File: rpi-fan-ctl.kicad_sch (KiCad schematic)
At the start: 21 parts, among them J2 Conn_01x05, Q4 NPN, U1 74LVC2G17, U2 74LVC2G17, U3 74LVC2G17

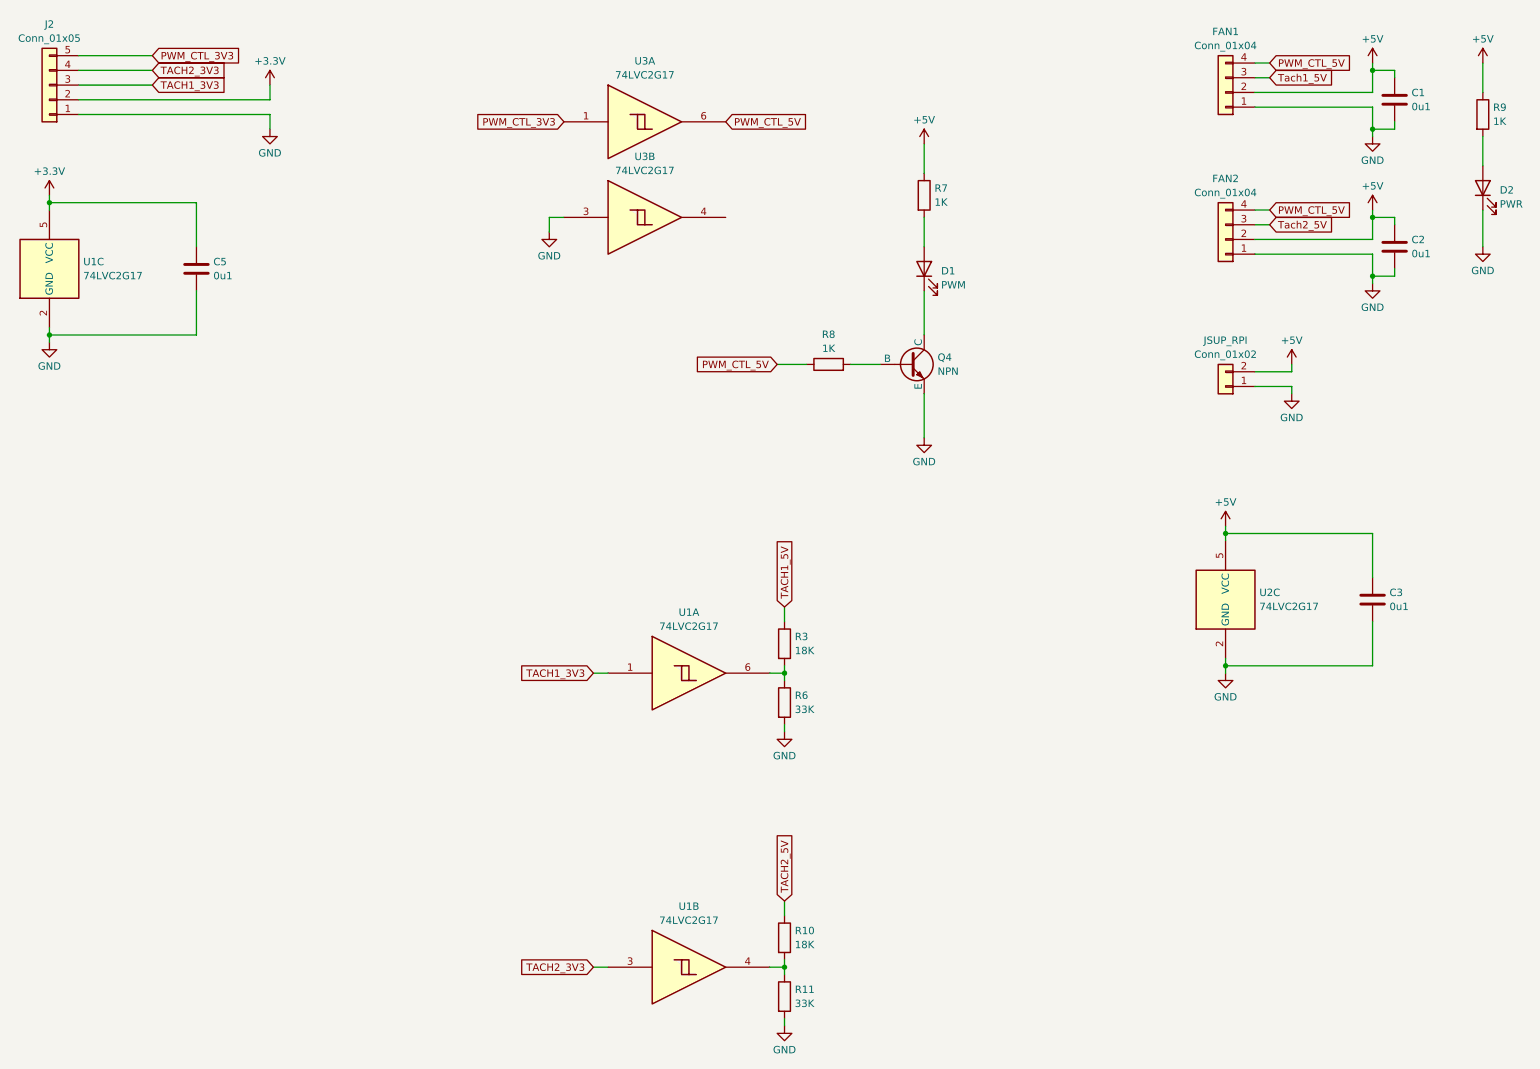
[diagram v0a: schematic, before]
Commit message: some routing progress
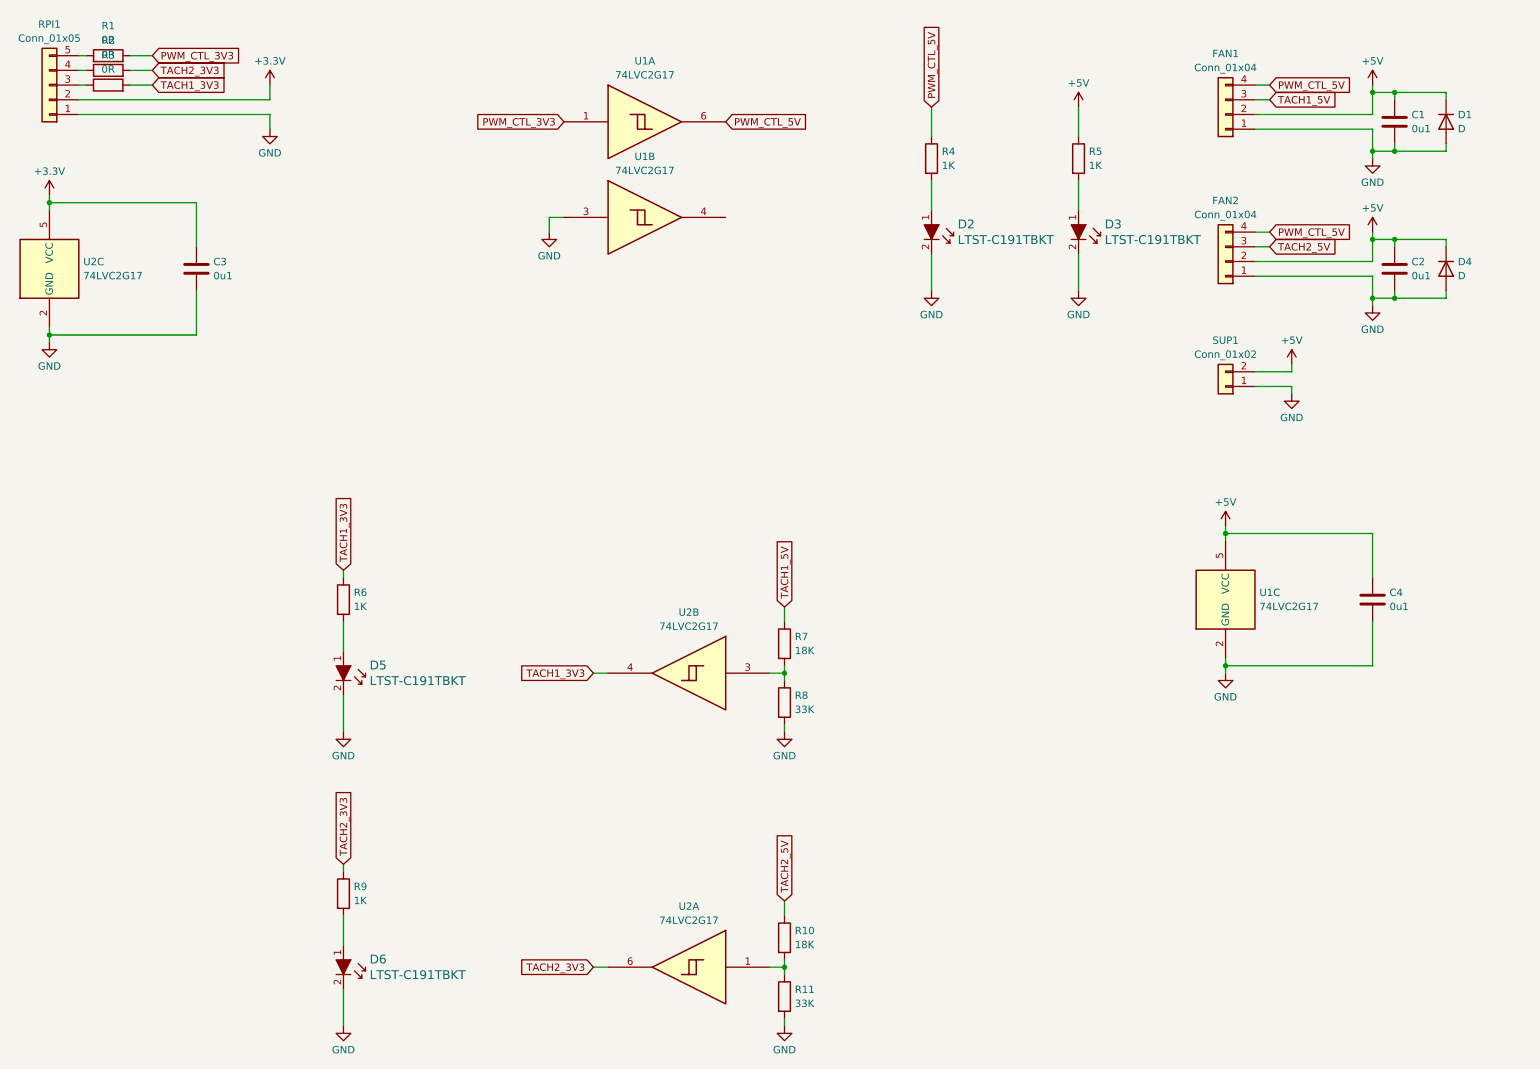
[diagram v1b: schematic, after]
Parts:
- removed D1: PWM, symbol Device:LED
- removed D2: PWR, symbol Device:LED
- removed Q4: NPN, symbol Simulation_SPICE:NPN
- removed R8: 1K, Resistor_SMD:R_0603_1608Metric_Pad0.98x0.95mm_HandSolder, symbol Device:R
- added D1: D, Diode_SMD:D_SOD-123F, symbol Device:D
- added D2, D3, D5, D6: LTST-C191TBKT, Diode_SMD:D_0402_1005Metric_Pad0.77x0.64mm_HandSolder, symbol J-Link-SWD-rescue:LTST-C191TBKT-dk_LED-Indication-Discrete
- added D4: D, Diode_SMD:D_SOD-123, symbol Device:D
- added R1, R2, R3: 0R, Resistor_SMD:R_0603_1608Metric_Pad0.98x0.95mm_HandSolder, symbol Device:R
- added R6, R9: 1K, Resistor_SMD:R_0603_1608Metric_Pad0.98x0.95mm_HandSolder, symbol Device:R
- FAN1, FAN2: footprint (none) -> Connector_PinHeader_2.54mm:PinHeader_1x04_P2.54mm_Horizontal
- RPI1: renamed from J2; footprint (none) -> Connector_PinHeader_2.54mm:PinHeader_1x05_P2.54mm_Vertical
- SUP1: renamed from JSUP_RPI; footprint (none) -> Connector_PinHeader_2.54mm:PinHeader_1x02_P2.54mm_Horizontal
- U1: renamed from U3; footprint Package_TO_SOT_SMD:SOT-363_SC-70-6_Handsoldering -> Package_TO_SOT_SMD:SOT-23-6_Handsoldering; DigiKey https://www.digikey.de/en/products/detail/texas-instruments/SN74LVC2G17DCKR/479737 -> https://www.digikey.de/en/products/detail/texas-instruments/SN74LVC2G17DBVR/479735
- U1: renamed from U2; footprint (none) -> Package_TO_SOT_SMD:SOT-23-6_Handsoldering; DigiKey (none) -> https://www.digikey.de/en/products/detail/texas-instruments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
- U2: renamed from U1; footprint Package_TO_SOT_SMD:SOT-363_SC-70-6_Handsoldering -> Package_TO_SOT_SMD:SOT-23-6_Handsoldering; DigiKey https://www.digikey.de/en/products/detail/texas-instruments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 -> (none)
- U2: renamed from U1; footprint (none) -> Package_TO_SOT_SMD:SOT-23-6_Handsoldering
- renumbered C5 to C3, C3 to C4, R7 to R4, R9 to R5, R3 to R7, R6 to R8
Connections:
- net Tach1_5V is gone; now on net TACH1_5V: FAN1.3 (Pin_3)
- net Tach2_5V is gone; now on net TACH2_5V: FAN2.3 (Pin_3)
- net +5V: now also D1.1 (K), D4.1 (K); no longer R4.1
- net GND: now also D1.2 (A), D2.2, D3.2, D4.2 (A), D5.2, D6.2
- net PWM_CTL_3V3: now also R1.2; no longer RPI1.5 (Pin_5)
- net PWM_CTL_5V: now also R4.1
- net TACH1_3V3: now also U2.4, R3.2, R6.1; no longer RPI1.3 (Pin_3), U2.1
- net TACH2_3V3: now also U2.6, R2.2, R9.1; no longer RPI1.4 (Pin_4), U2.3
- net at R7.2, R8.1: now also U2.3; no longer U2.6
- net at R5.2: now also D3.1
- net at R10.2, R11.1: now also U2.1; no longer U2.4
- net at R4.2: now also D2.1
- new net: D5.1, R6.2
- new net: R1.1, RPI1.5 (Pin_5)
- new net: R3.1, RPI1.3 (Pin_3)
- new net: R2.1, RPI1.4 (Pin_4)
- new net: D6.1, R9.2
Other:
- moved on the sheet: C1, C2, FAN1, FAN2, R4, R5, U2A, U2B
